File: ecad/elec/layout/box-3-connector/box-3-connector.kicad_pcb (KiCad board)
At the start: 2 copper layers, 72.5 x 7.9 mm, 2 parts

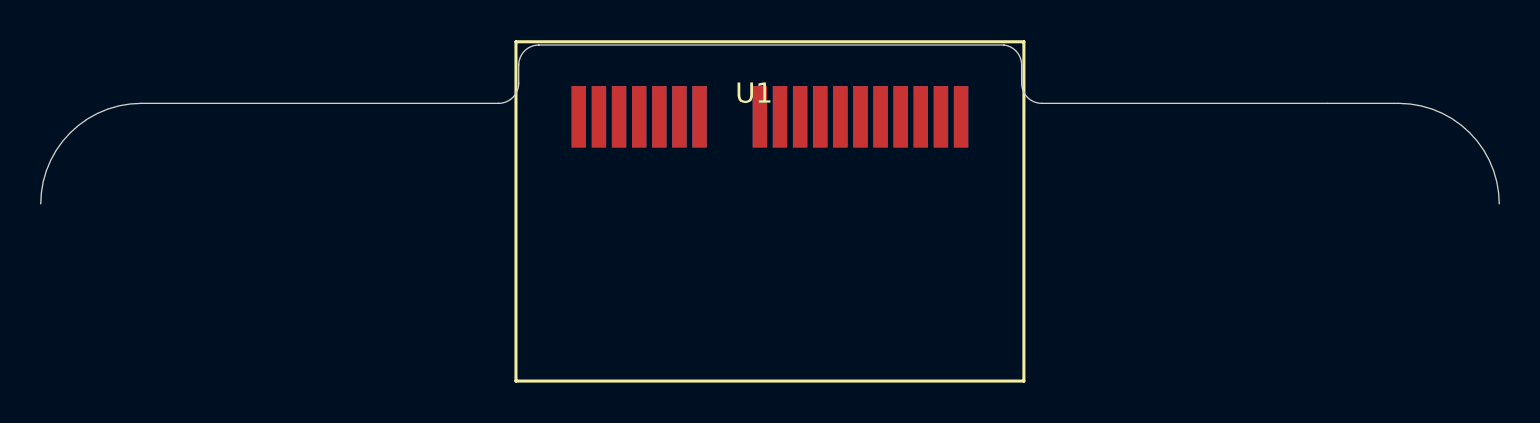
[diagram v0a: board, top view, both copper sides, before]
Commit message: update layouts
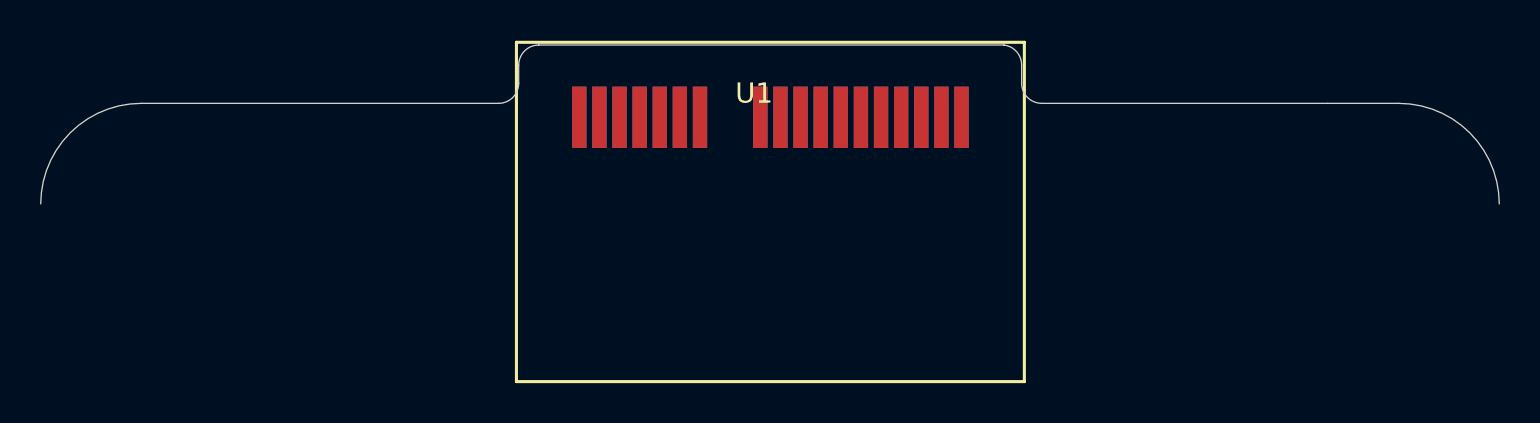
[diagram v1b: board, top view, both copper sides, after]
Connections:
- net cc4484681-gnd renamed conn-gnd
